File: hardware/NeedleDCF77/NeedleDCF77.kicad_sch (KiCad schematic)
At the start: 53 parts, among them J1 USB_C_Receptacle_USB2.0

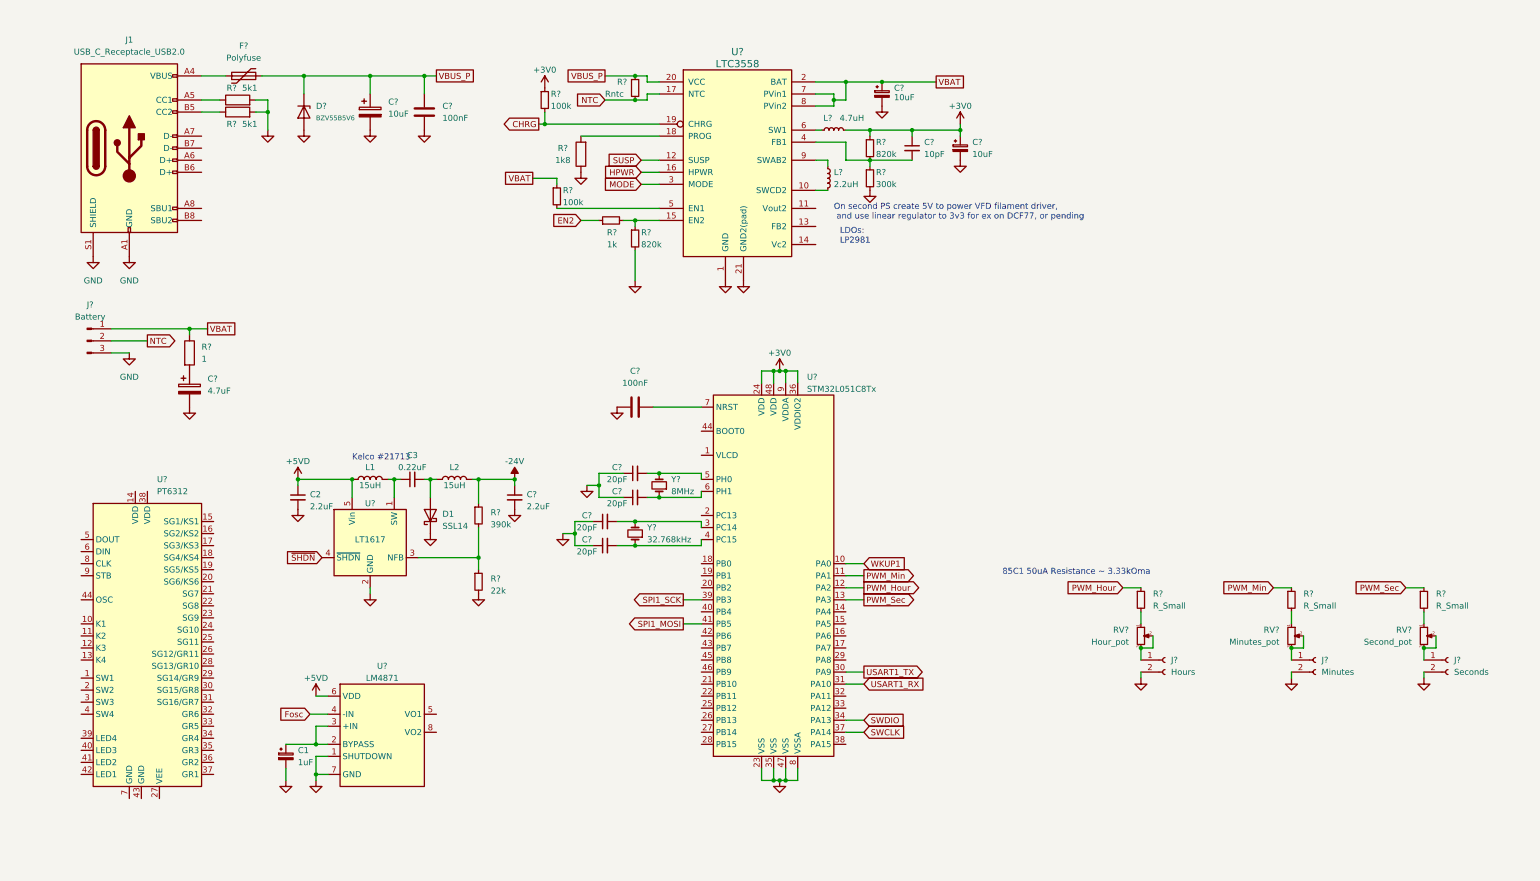
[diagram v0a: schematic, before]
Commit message: Implement VFD circuit
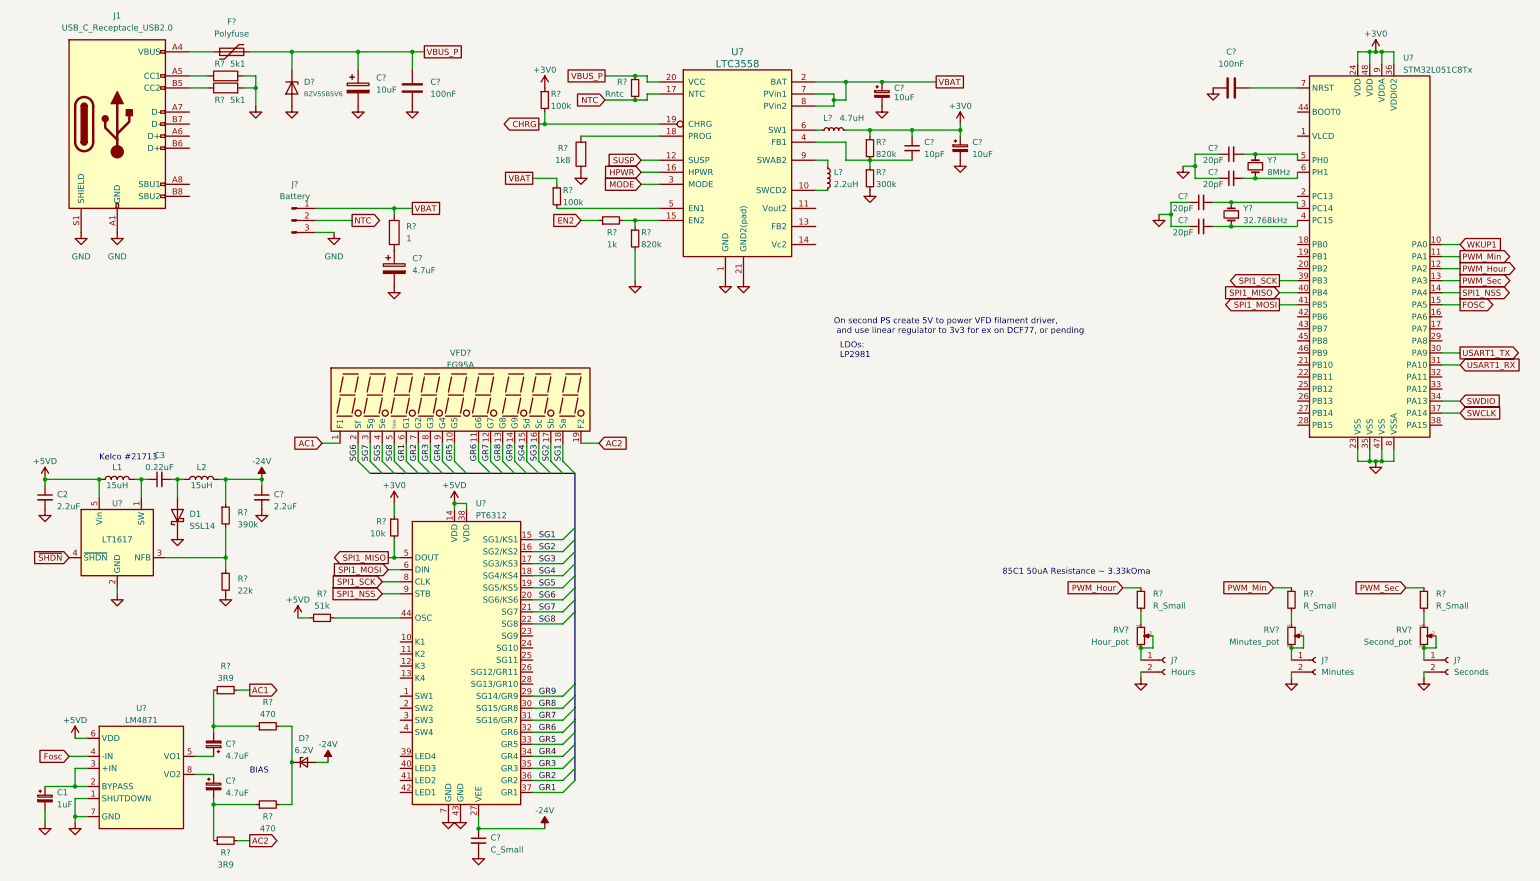
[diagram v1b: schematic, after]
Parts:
- added C?: C_Small, symbol Device:C_Small
- added C? (x2): 4.7uF, symbol Device:C_Polarized_Small
- added D?: 6.2V, symbol Device:D_Zener_Small
- added R?: 10k, symbol Device:R_Small
- added R? (x2): 470, symbol Device:R_Small
- added R? (x2): 3R9, symbol Device:R_Small
- added R?: 51k, symbol Device:R_Small
- added VFD?: FG95A, VFD:FG95A, symbol VFD:FG95A
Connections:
- net +3V0: now also R?.1
- net +5VD: now also U?.14 (VDD), U?.38 (VDD), R?.1
- net -24V: now also U?.27 (VEE), C?.1, D?.2 (A)
- net GND: now also U?.43 (GND), U?.7 (GND), C?.2
- net SPI1_MOSI: now also U?.6 (DIN)
- net SPI1_SCK: now also U?.8 (CLK)
- net SG1: now reaches U?.15 (SG1/KS1)
- net SG1: now also VFD?.18 (Sa)
- net SG2: now reaches U?.16 (SG2/KS2)
- net SG2: now also VFD?.17 (Sb)
- net SG3: now reaches U?.17 (SG3/KS3)
- net SG3: now also VFD?.16 (Sc)
- net SG4: now reaches U?.18 (SG4/KS4)
- net SG4: now also VFD?.15 (Sd)
- net SG5: now reaches U?.19 (SG5/KS5)
- net SG5: now also VFD?.4 (Se)
- net SG6: now reaches U?.20 (SG6/KS6)
- net SG6: now also VFD?.2 (Sf)
- net SG7: now reaches U?.21 (SG7)
- net SG7: now also VFD?.3 (Sg)
- net SG8: now reaches U?.22 (SG8)
- net SG8: now also VFD?.5 (Sdot)
- net GR9: now reaches U?.29 (SG14/GR9)
- net GR9: now also VFD?.14 (G9)
- net GR8: now reaches U?.30 (SG15/GR8)
- net GR8: now also VFD?.13 (G8)
- net GR7: now reaches U?.31 (SG16/GR7)
- net GR7: now also VFD?.12 (G7)
- net GR6: now reaches U?.32 (GR6)
- net GR6: now also VFD?.11 (G6)
- net GR5: now reaches U?.33 (GR5)
- net GR5: now also VFD?.10 (G5)
- net GR4: now reaches U?.34 (GR4)
- net GR4: now also VFD?.9 (G4)
- net GR3: now reaches U?.35 (GR3)
- net GR3: now also VFD?.8 (G3)
- net GR2: now reaches U?.36 (GR2)
- net GR2: now also VFD?.7 (G2)
- net GR1: now reaches U?.37 (GR1)
- net GR1: now also VFD?.6 (G1)
- net at U?.44 (OSC): now also R?.2
- net SPI1_MISO: now reaches U?.5 (DOUT)
- net SPI1_MISO: now also U?.40 (PB4), R?.2
- net SPI1_NSS: now reaches U?.9 (STB)
- net SPI1_NSS: now also U?.14 (PA4)
- net FOSC: now reaches U?.15 (PA5)
- net at U?.5 (VO1): now also C?.1
- net at U?.8 (VO2): now also C?.1
- new net: C?.2, R?.1, R?.1 (x2)
- new net: D?.1 (K), R?.2, R?.2
- new net AC1: R?.2, VFD?.1 (F1)
- new net AC2: R?.2, VFD?.19 (F2)
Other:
- note added: "BIAS"
- moved on the sheet: C1, C2, C3, C?, D1, D?, F?, J1, J?, L1, L2, R?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
